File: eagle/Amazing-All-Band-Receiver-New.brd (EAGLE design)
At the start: 33 x 17.8 mm, 20 parts, among them T1 2N2907, T2 2N2907

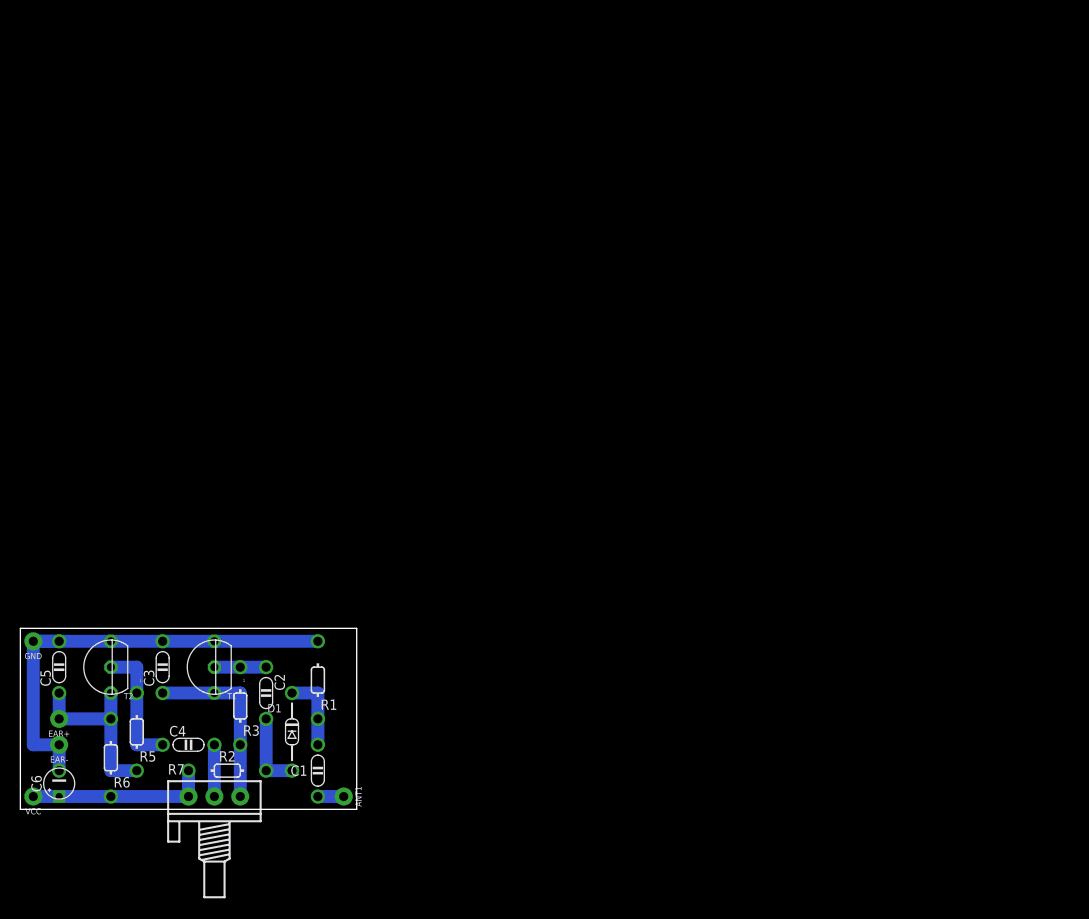
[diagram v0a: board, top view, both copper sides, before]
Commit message: ...
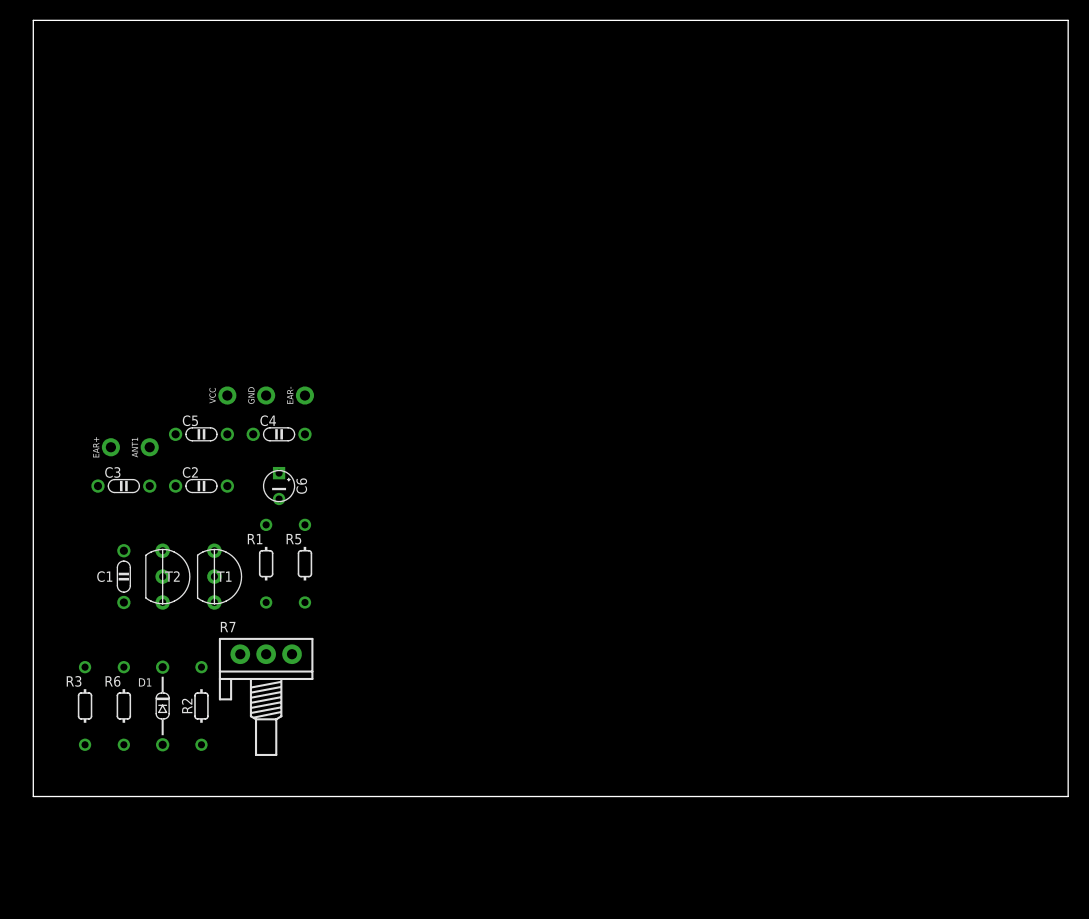
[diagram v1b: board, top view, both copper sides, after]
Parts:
- T1, T2: value 2N2907 -> BC547; device t:TO92 -> t:TO92-CBE
- moved VCC 43.7 mm to (19.1, 39.4), turned to 0 degrees
- moved EAR- 41.9 mm to (26.7, 39.4), turned to 0 degrees
- moved ANT1 39.2 mm to (11.4, 34.3), turned to 0 degrees
- moved C6 36.3 mm to (24.1, 30.5), turned to 0 degrees
- moved GND 33.2 mm to (22.9, 39.4), turned to 0 degrees
- moved C4 31.8 mm to (24.1, 35.6)
- moved EAR+ 27.1 mm to (7.62, 34.3), turned to 0 degrees
- moved C1 26.9 mm to (8.89, 21.6)
- moved C5 26.8 mm to (16.5, 35.6), turned to 0 degrees
- moved R5 23.3 mm to (26.7, 22.9), turned to 0 degrees
- moved C2 21.3 mm to (16.5, 30.5), turned to 0 degrees
- moved C3 18.2 mm to (8.89, 30.5), turned to 0 degrees
- moved R3 15.2 mm to (5.08, 8.89), turned to 0 degrees
- moved R7 14.9 mm to (22.9, 14.0)
- moved D1 13.0 mm to (12.7, 8.89)
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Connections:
- net GND: now also T1.E, T2.E; no longer T1.3, T2.3
- net I1: now also T1.B; no longer T1.2
- net I2: now also T2.B; no longer T2.2
- net O1: now also T1.C; no longer T1.1
- net O2: now also T2.C; no longer T2.1
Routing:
- net GND: track 45.7 -> 0.00 mm, vias 1 -> 0
- net VCC: track 17.8 -> 0.00 mm
- net O2: track 17.8 -> 0.00 mm
- net O1: track 17.8 -> 0.00 mm
- net I2: track 12.7 -> 0.00 mm
- net AC: track 7.62 -> 0.00 mm
- net DC: track 7.62 -> 0.00 mm
- net VO1: track 5.08 -> 0.00 mm
- net I1: track 5.08 -> 0.00 mm
- net ANT: track 2.54 -> 0.00 mm
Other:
- board size 33 x 17.8 mm -> 101.6 x 76.2 mm
